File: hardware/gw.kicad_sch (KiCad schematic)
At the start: 21 parts, among them J1 USB_OTG, J2 Conn_01x04, U1 ESP-12F, U2 Ai-Thinker-Ra-02, U3 AMS1117-3.3

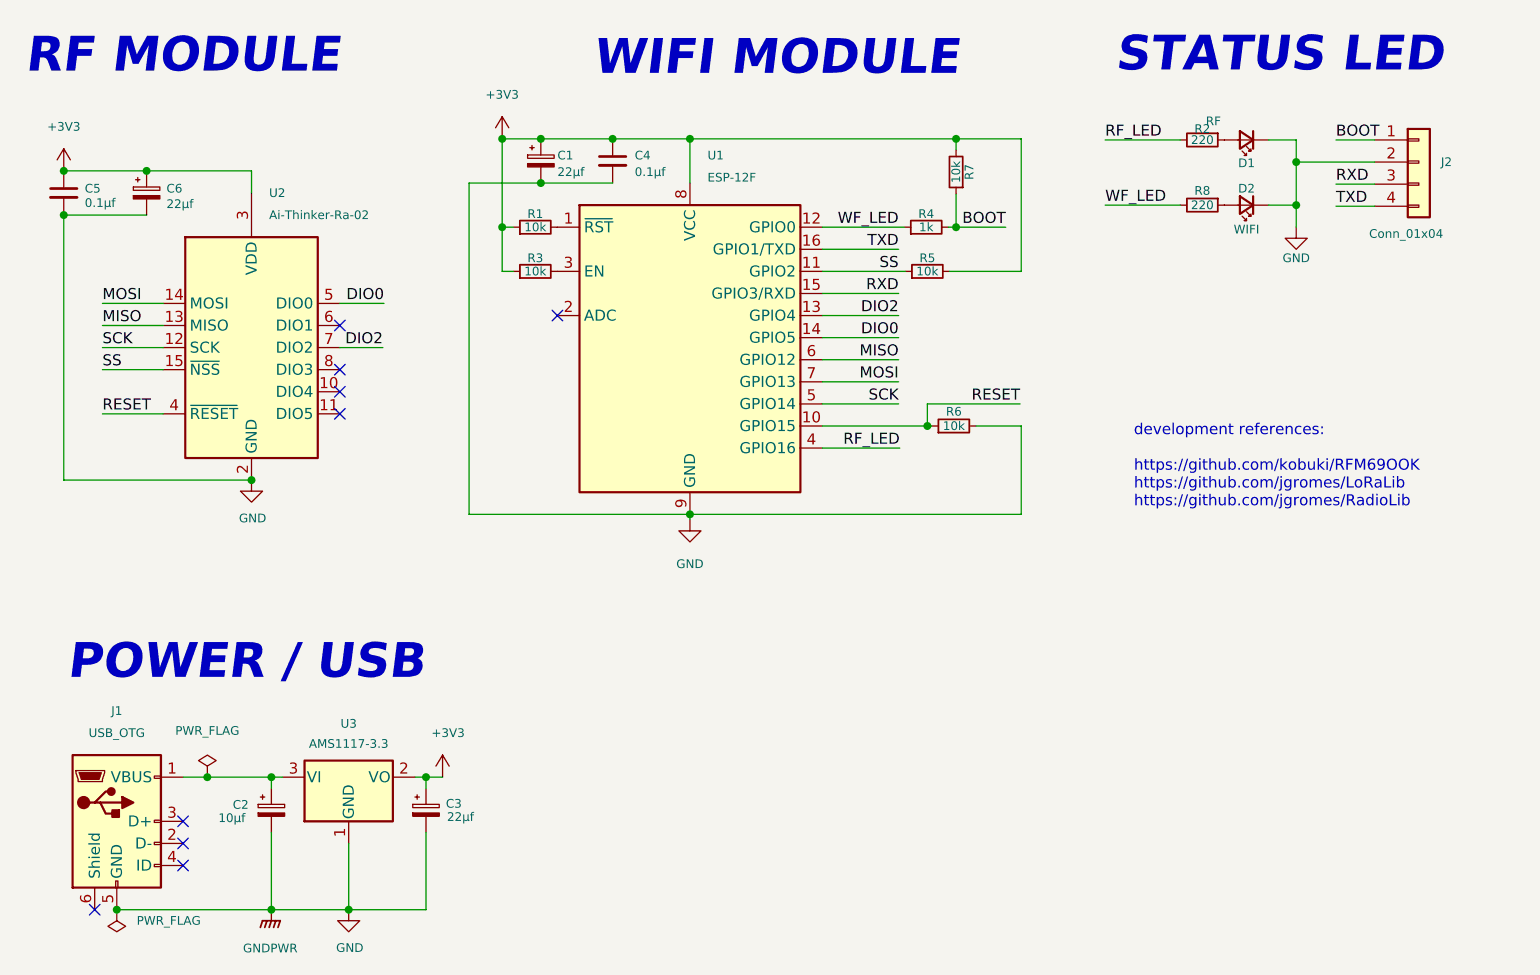
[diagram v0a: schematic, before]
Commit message: Cleanup sch
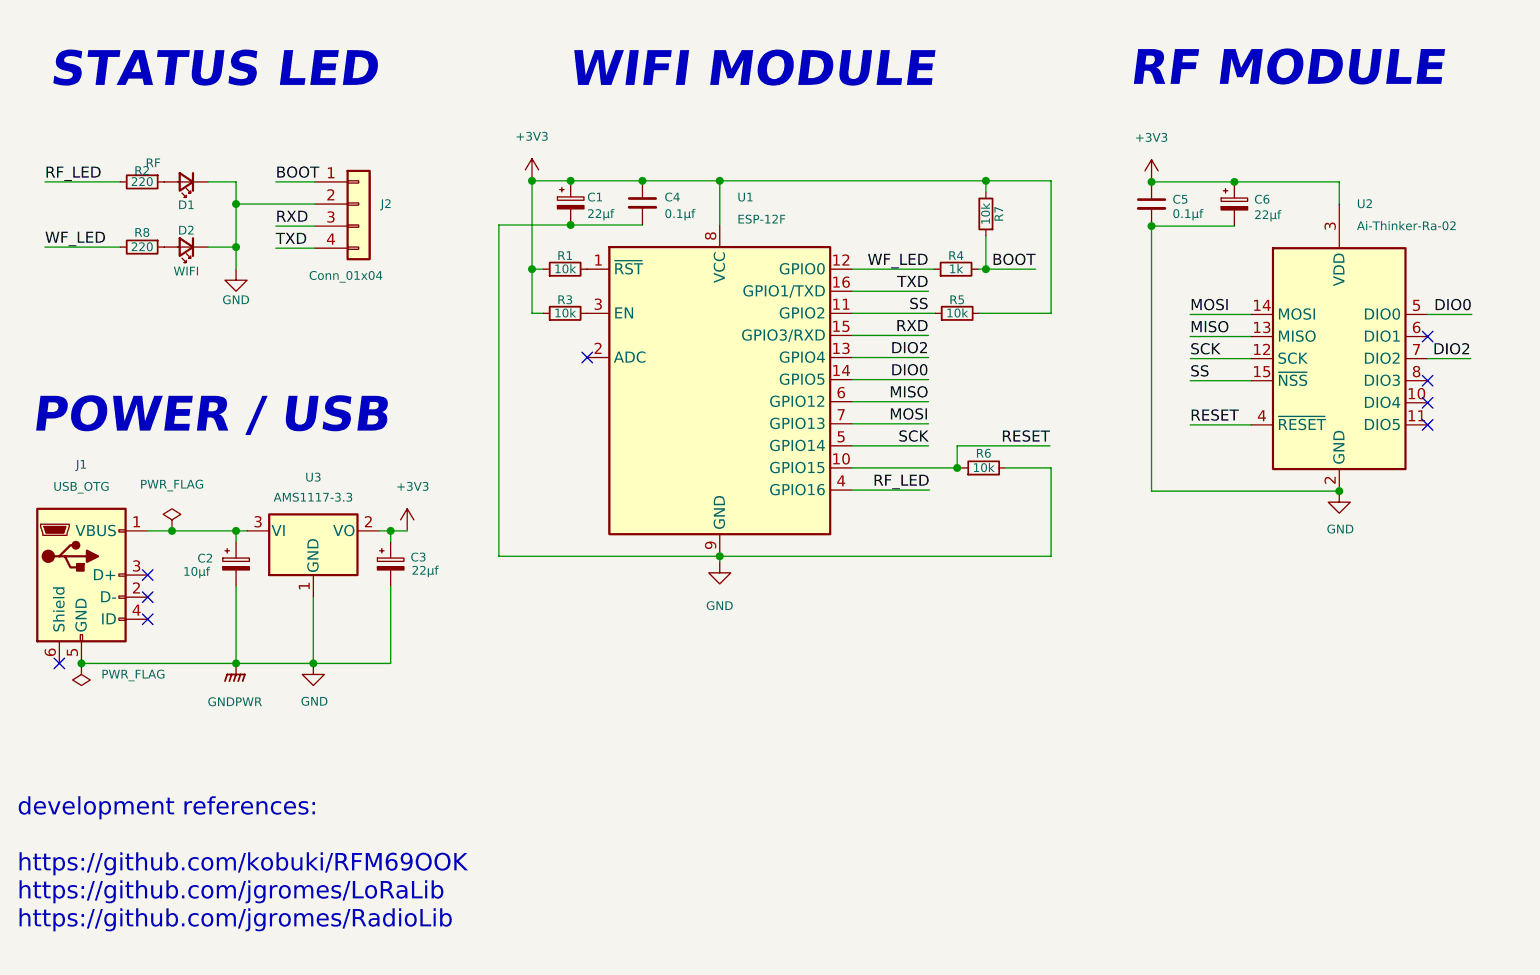
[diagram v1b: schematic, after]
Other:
- moved on the sheet: C1, C2, C3, C4, C5, C6, D1, D2, J1, J2, R1, R2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
